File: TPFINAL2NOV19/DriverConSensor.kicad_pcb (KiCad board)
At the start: 2 copper layers, 77 x 67 mm, 53 parts, among them J1 PULS1, J2 PULS2, J3 MotorT2, J4 MotorT1, J5 VIn+12, J6 Contac12V, J7 GND, K1 Switch de Encendido, K2 FRS10CS10-12V, K3 FRS10CS10-12V, Q1 BC337, Q2 BC337, SW1 SW_DIP_x06, U1 PIC12F675-IP, U2 L78L05_TO92, U3 ACS714T-30A

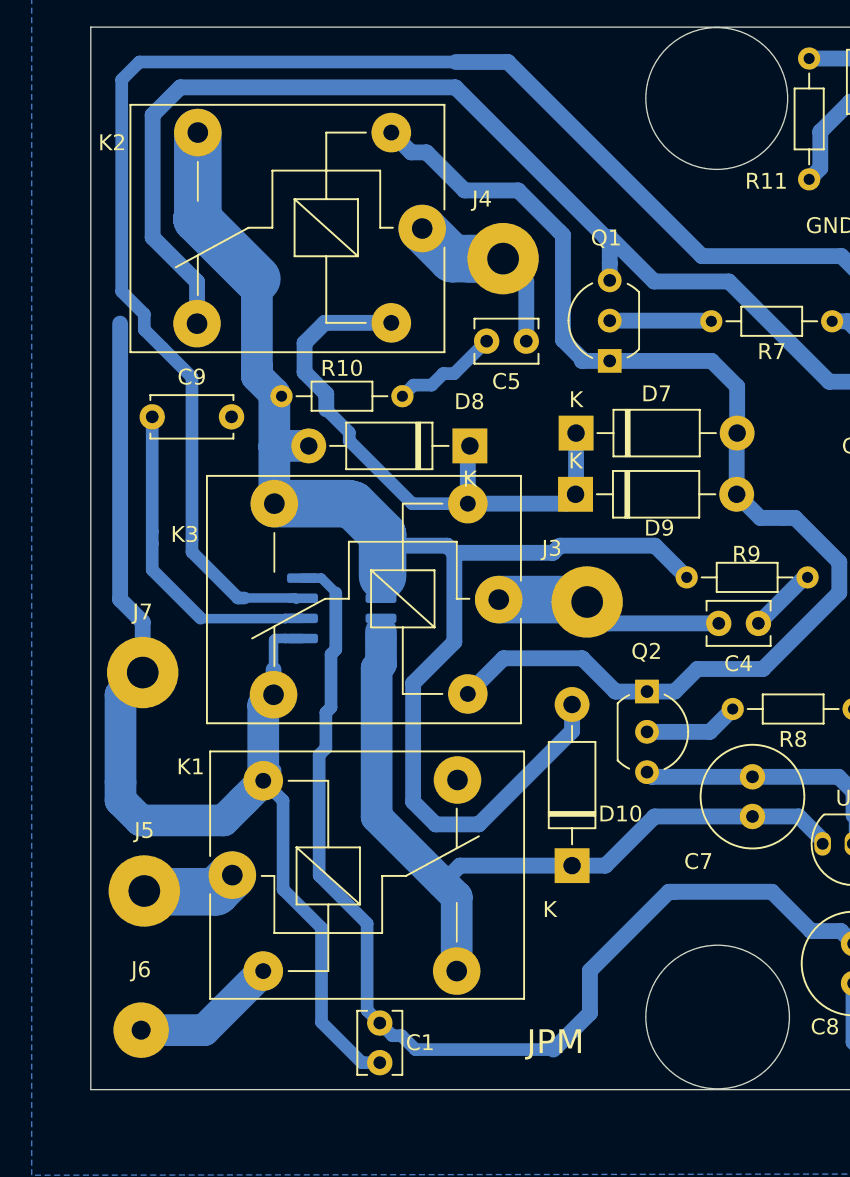
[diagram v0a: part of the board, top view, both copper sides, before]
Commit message: PCB
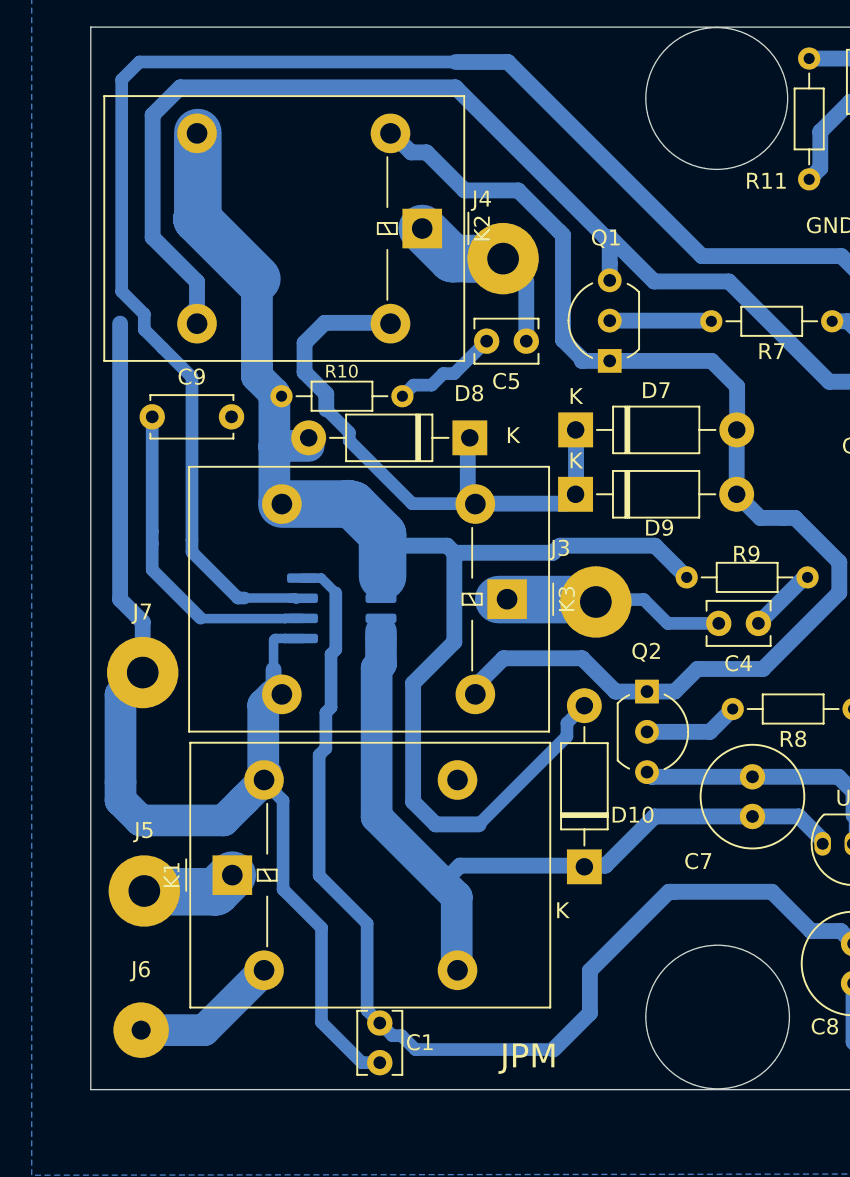
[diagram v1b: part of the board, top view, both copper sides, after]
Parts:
- K1, K2, K3: footprint Relay_THT:Relay_SPDT_SANYOU_SRD_Series_Form_C -> Relay_THT:Relay_SPDT_Omron-G5LE-1
- moved D10 0.78 mm to (144.1, 116.0)
- moved J3 0.55 mm to (144.8, 99.2)
- moved K3 0.53 mm to (139.2, 99.1), turned to 270 degrees
- moved D8 0.51 mm to (136.9, 88.9)
- moved D7 0.20 mm to (143.6, 88.4)
- turned K1 to 90 degrees
- turned K2 to 270 degrees
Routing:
- net Net-(C4-Pad2): track 14.5 -> 16.0 mm
